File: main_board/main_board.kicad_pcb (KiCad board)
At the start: 2 copper layers, 95.9 x 90.2 mm, 42 parts, among them J1 Conn_02x20_Odd_Even, J2 AudioJack2_Ground_SwitchT, J3 USB_C_Receptacle_USB2.0_14P, J4 Conn_01x03, J8 Conn_01x02, SW1 SW_SPST, SW3 SW_SPST, U1 RP2040, U2 W25Q128JVS, Y2 ASE-12MHz

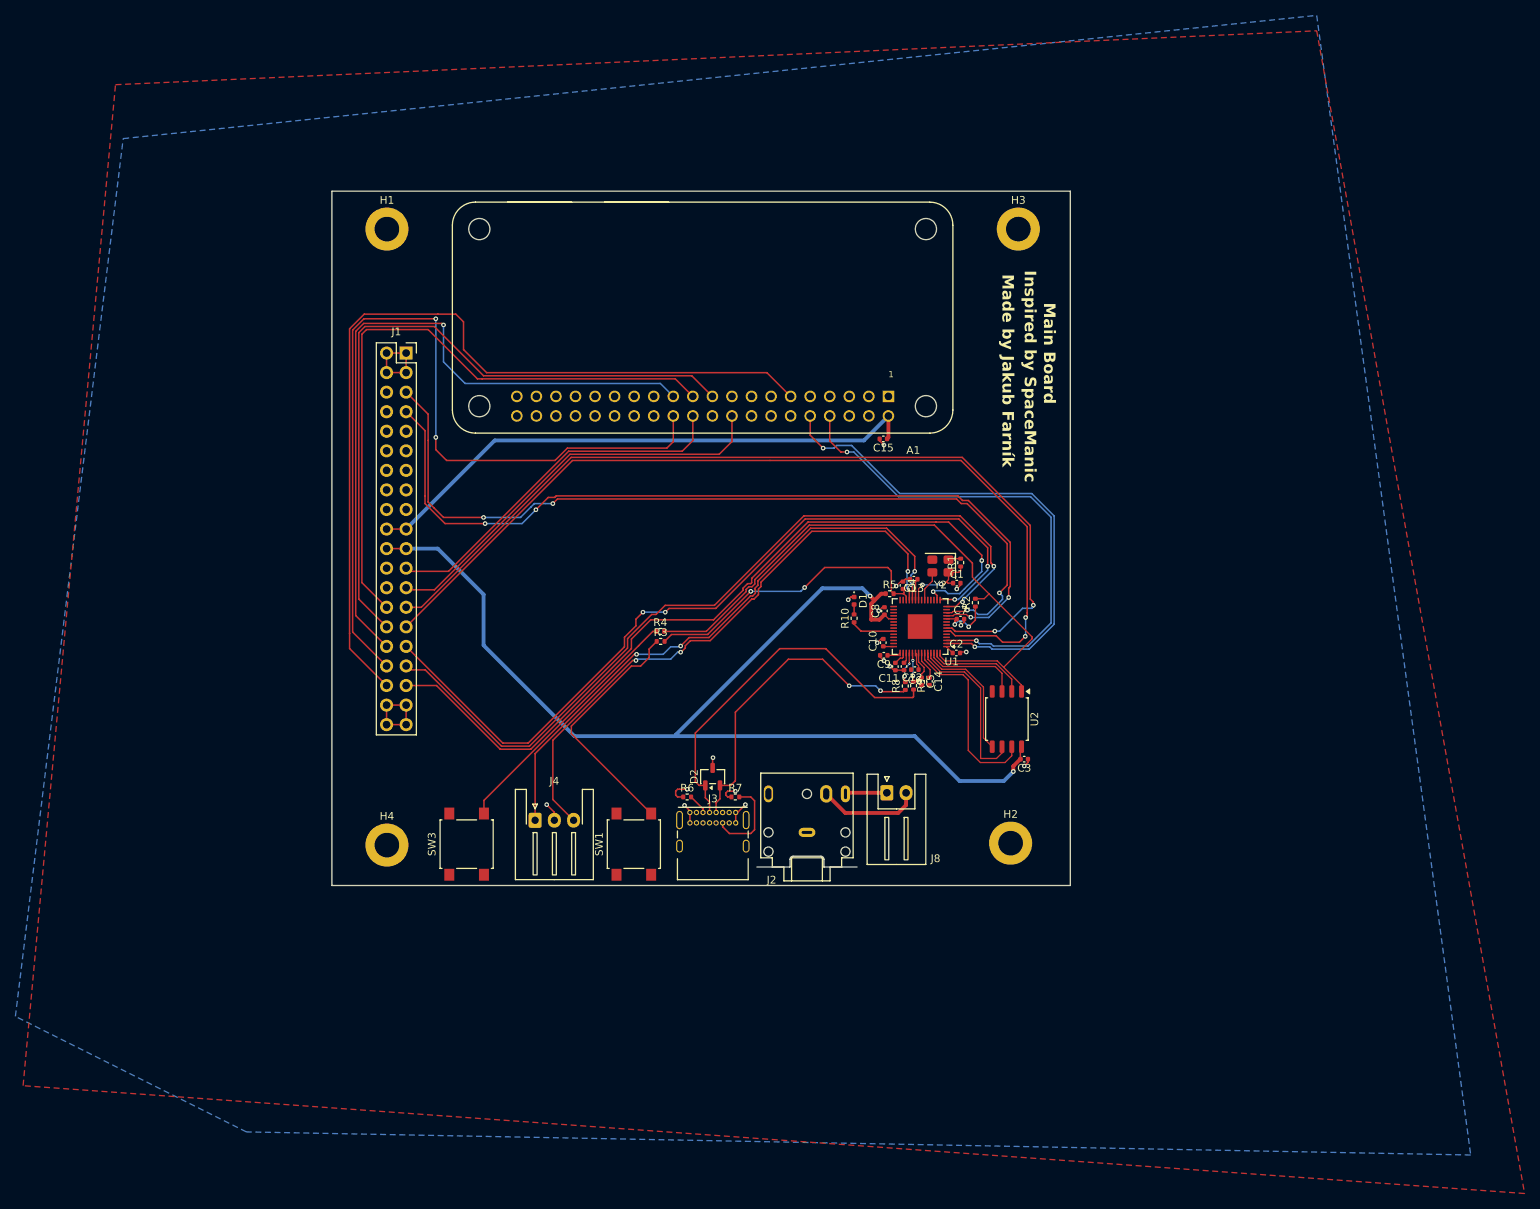
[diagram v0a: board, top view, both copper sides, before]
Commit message: main board complete
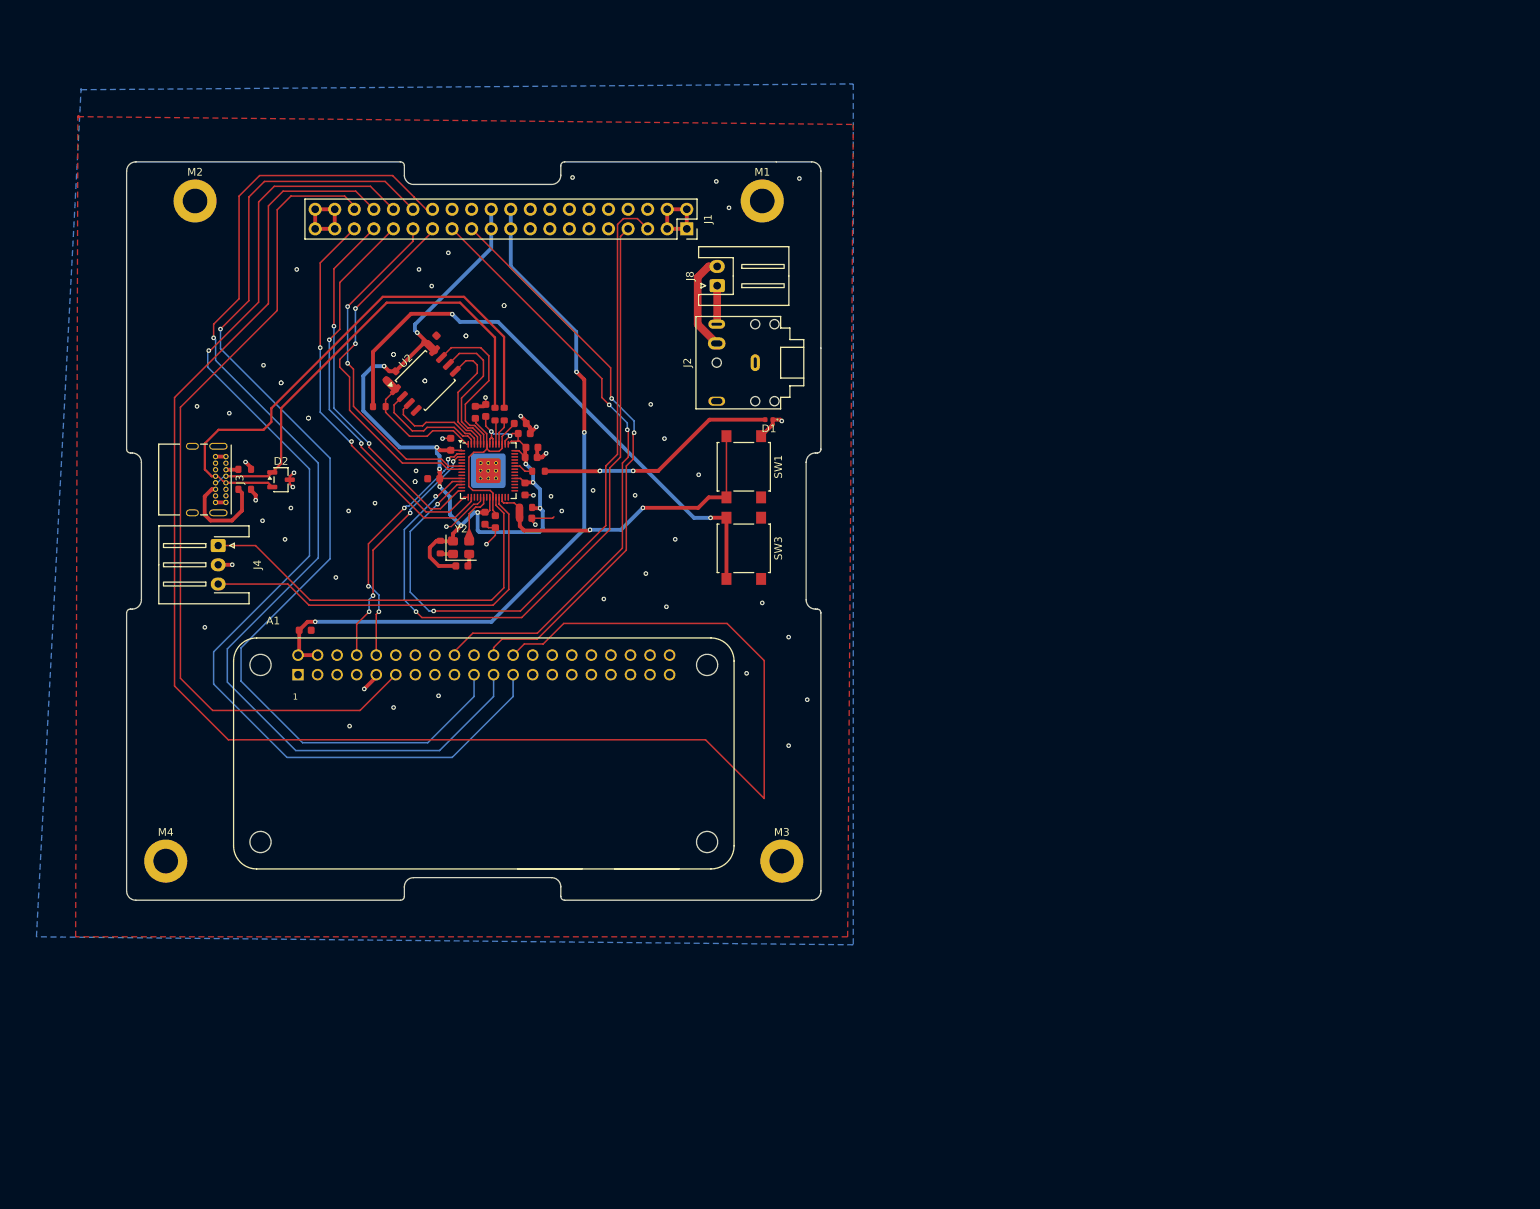
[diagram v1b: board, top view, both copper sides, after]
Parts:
- removed C1: 1uF, Capacitor_SMD:C_0402_1005Metric
- removed C10, C5, C6, C7, C8, C9: 100nF, Capacitor_SMD:C_0402_1005Metric
- removed H1, H2, H3, H4: MountingHole_Pad, MountingHole:MountingHole_3.2mm_M3_DIN965_Pad
- removed R10: 1K, Resistor_SMD:R_0402_1005Metric
- removed R8, R9: 27.4R, Resistor_SMD:R_0402_1005Metric
- removed U1: RP2040, Package_DFN_QFN:QFN-56-1EP_7x7mm_P0.4mm_EP3.2x3.2mm
- added C16: 100nF, PCM_JLCPCB:C_0603, F.Cu at (89.6, 97.9)
- added C17: 100nF, PCM_JLCPCB:C_0603, F.Cu at (106.1, 60.1)
- added C18: 100nF, PCM_JLCPCB:C_0603, F.Cu at (119.0, 75.4)
- added C19: 100nF, PCM_JLCPCB:C_0603, F.Cu at (106.3, 78.2)
- added C20: 100nF, PCM_JLCPCB:C_0603, F.Cu at (113.1, 69.3)
- added C21: 100nF, PCM_JLCPCB:C_0603, F.Cu at (118.2, 79.5)
- added C22: 100nF, PCM_JLCPCB:C_0603, F.Cu at (119.1, 74.1)
- added M1: MountingHole_Pad, MountingHole:MountingHole_3.2mm_M3_DIN965_Pad, F.Cu at (149.0, 42.1)
- added M2: MountingHole_Pad, MountingHole:MountingHole_3.2mm_M3_DIN965_Pad, F.Cu at (75.3, 42.1)
- added M3: MountingHole_Pad, MountingHole:MountingHole_3.2mm_M3_DIN965_Pad, F.Cu at (151.5, 127.8)
- added M4: MountingHole_Pad, MountingHole:MountingHole_3.2mm_M3_DIN965_Pad, F.Cu at (71.5, 127.8)
- added R11: 5.1kΩ, PCM_JLCPCB:R_0603, F.Cu at (81.8, 77.0)
- added R12: 5.1kΩ, PCM_JLCPCB:R_0603, F.Cu at (81.8, 79.6)
- added U3: RP2040, PCM_JLCPCB:QFN-56-1EP_7x7mm_P0.4mm_EP3.2x3.2mm_ThermalVias, F.Cu at (113.4, 77.1)
- C11, C15, C2: footprint Capacitor_SMD:C_0402_1005Metric -> PCM_JLCPCB:C_0603
- C12: value 1u -> 100nF; footprint Capacitor_SMD:C_0402_1005Metric -> PCM_JLCPCB:C_0603
- C13, C14: value 100n -> 100nF; footprint Capacitor_SMD:C_0402_1005Metric -> PCM_JLCPCB:C_0603
- C3: value 100nF -> 1uF; footprint Capacitor_SMD:C_0402_1005Metric -> PCM_JLCPCB:C_0603
- C4: value C -> 1uF; footprint Capacitor_SMD:C_0402_1005Metric -> PCM_JLCPCB:C_0603
- R1, R5: value 10K -> 27Ω; footprint Resistor_SMD:R_0402_1005Metric -> PCM_JLCPCB:R_0603
- R2: value 10K -> 10kΩ; footprint Resistor_SMD:R_0402_1005Metric -> PCM_JLCPCB:R_0603
- R3, R4: value 1K -> 10kΩ; footprint Resistor_SMD:R_0402_1005Metric -> PCM_JLCPCB:R_0603
- R6, R7: value 5.1K -> 1kΩ; footprint Resistor_SMD:R_0402_1005Metric -> PCM_JLCPCB:R_0603
- moved U2 87.4 mm to (105.2, 65.4), turned to 45 degrees
- moved C3 77.2 mm to (110.0, 89.5), turned to 0 degrees
- moved J3 75.9 mm to (79.3, 75.3), turned to -90 degrees
- moved R2 69.9 mm to (107.2, 87.1), turned to -90 degrees
- moved J8 69.4 mm to (143.1, 53.1), turned to 90 degrees
- moved C14 69.4 mm to (108.5, 73.7), turned to 90 degrees
- moved R7 68.6 mm to (99.3, 68.8)
- moved D2 68.0 mm to (86.5, 78.3), turned to 0 degrees
- moved C12 64.7 mm to (111.7, 69.6), turned to 90 degrees
- moved R1 63.5 mm to (114.3, 69.8), turned to -90 degrees
- moved Y2 62.3 mm to (109.9, 87.1), turned to 0 degrees
- moved J2 61.4 mm to (148.1, 63.1), turned to 90 degrees
- moved C2 58.6 mm to (118.3, 83.3), turned to 180 degrees
- moved C11 56.9 mm to (118.1, 72.3), turned to 0 degrees
- moved R5 55.2 mm to (115.5, 69.8), turned to -90 degrees
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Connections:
- C14 pad 1: +1V1 -> +3V3
- C15 pad 1: +5V -> +3V3
- C2 pad 1: +3V3 -> GND
- C2 pad 2: GND -> RUN
- C3 pad 1: GND -> +3V3
- C3 pad 2: +3V3 -> GND
- C4 pad 1: GND -> +1V1
- C4 pad 2: RUN -> GND
- R1 pad 1: +3V3 -> USB_D+
- R1 pad 2: Net-(Y2-EN) -> Net-(U3-USB_DP)
- R2 pad 2: QSPLI_SS -> Net-(Y2-EN)
- R3 pad 1: Net-(SW1-B) -> +3V3
- R3 pad 2: RUN -> QSPLI_SS
- R4 pad 1: Net-(SW3-B) -> +3V3
- R4 pad 2: QSPLI_SS -> RUN
- R5 pad 1: +3V3 -> USB_D-
- R5 pad 2: RUN -> Net-(U3-USB_DM)
- R6 pad 1: GND -> GPIO25
- R6 pad 2: Net-(J3-CC1) -> Net-(D1-A)
- R7 pad 1: GND -> Net-(SW3-B)
- R7 pad 2: Net-(J3-CC2) -> QSPLI_SS
- SW1 pad 2: Net-(SW1-B) -> RUN
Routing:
- net NSS: track 109.6 -> 219.7 mm, vias 2 -> 0
- net SDA: track 118.6 -> 44.2 mm
- net SCL: track 116.3 -> 46.8 mm
- net QSPLI_SS: track 81.9 -> 18.2 mm
- net MISO: track 83.6 -> 147.1 mm, vias 0 -> 1
- net LED_WARN: track 106.4 -> 48.7 mm
- net LED_ERROR: track 106.3 -> 51.7 mm, vias 4 -> 2
- net SCK: track 91.0 -> 144.6 mm
- net LED_SUCCESS: track 104.5 -> 52.7 mm
- net MOSI: track 89.7 -> 137.6 mm, vias 0 -> 1
- net +3V3: track 173.9 -> 128.1 mm, vias 6 -> 12
- net Net-(SW3-B): track 33.2 -> 74.0 mm, vias 0 -> 2
- net ZERO_RX: track 68.5 -> 32.8 mm, vias 2 -> 4
- net ZERO_TX: track 64.9 -> 31.7 mm, vias 2 -> 4
- net Net-(SW1-B): track 31.9 -> 0.00 mm
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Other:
- board size 95.9 x 90.2 mm -> 90.2 x 95.9 mm
- board text added: "JLCJLCJLCJLC"
- board text removed: "Inspired by SpaceManic"
- board text removed: "Made by Jakub Farník"
- board text removed: "Main Board"
